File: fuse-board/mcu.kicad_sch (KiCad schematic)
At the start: 33 parts, among them IC1 TMUX1308QPWRQ1, J1 FTSH-107-01-F-DV-K-P-TR, SW1 Y97KT23B5NAFP, U1 STM32G441KBTx, Y1 ECS-240-8-37B-CKY-TR

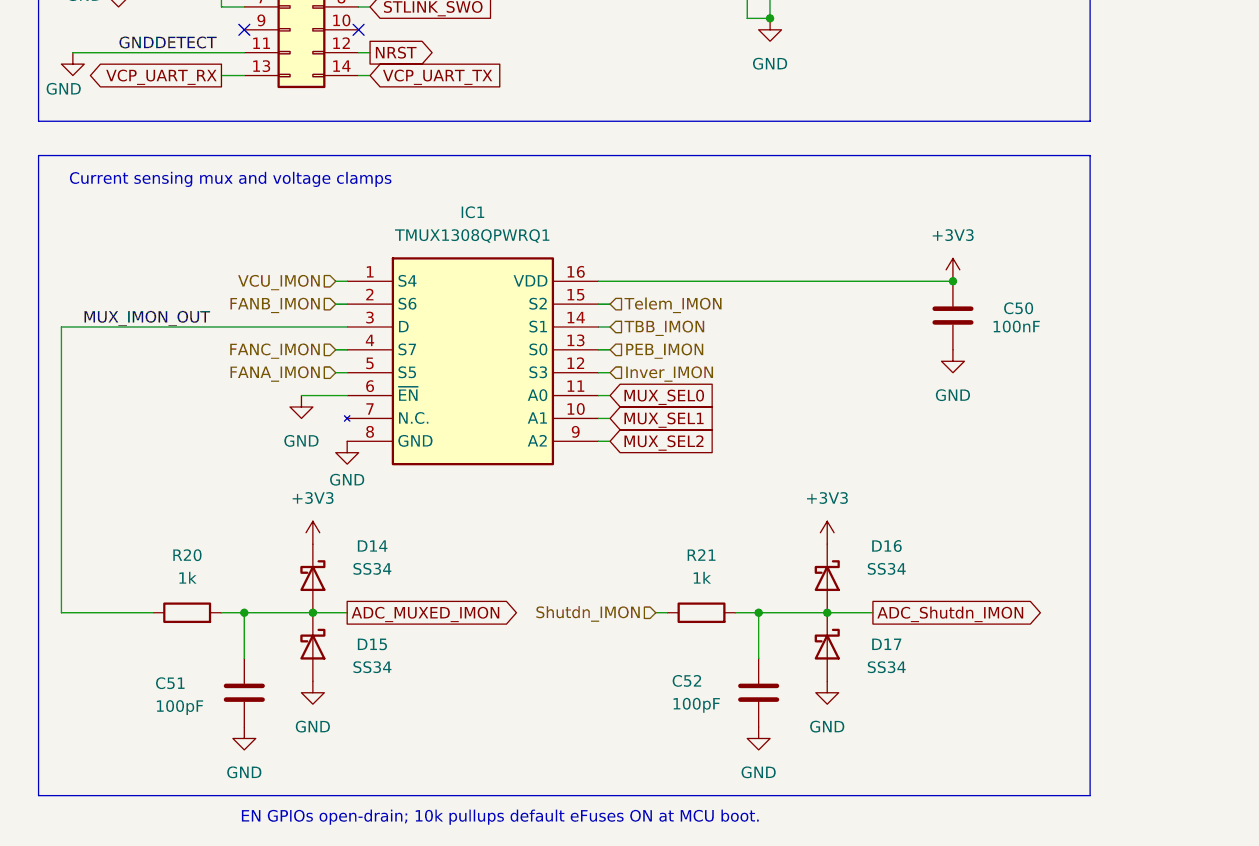
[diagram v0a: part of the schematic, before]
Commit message: update tmux1308
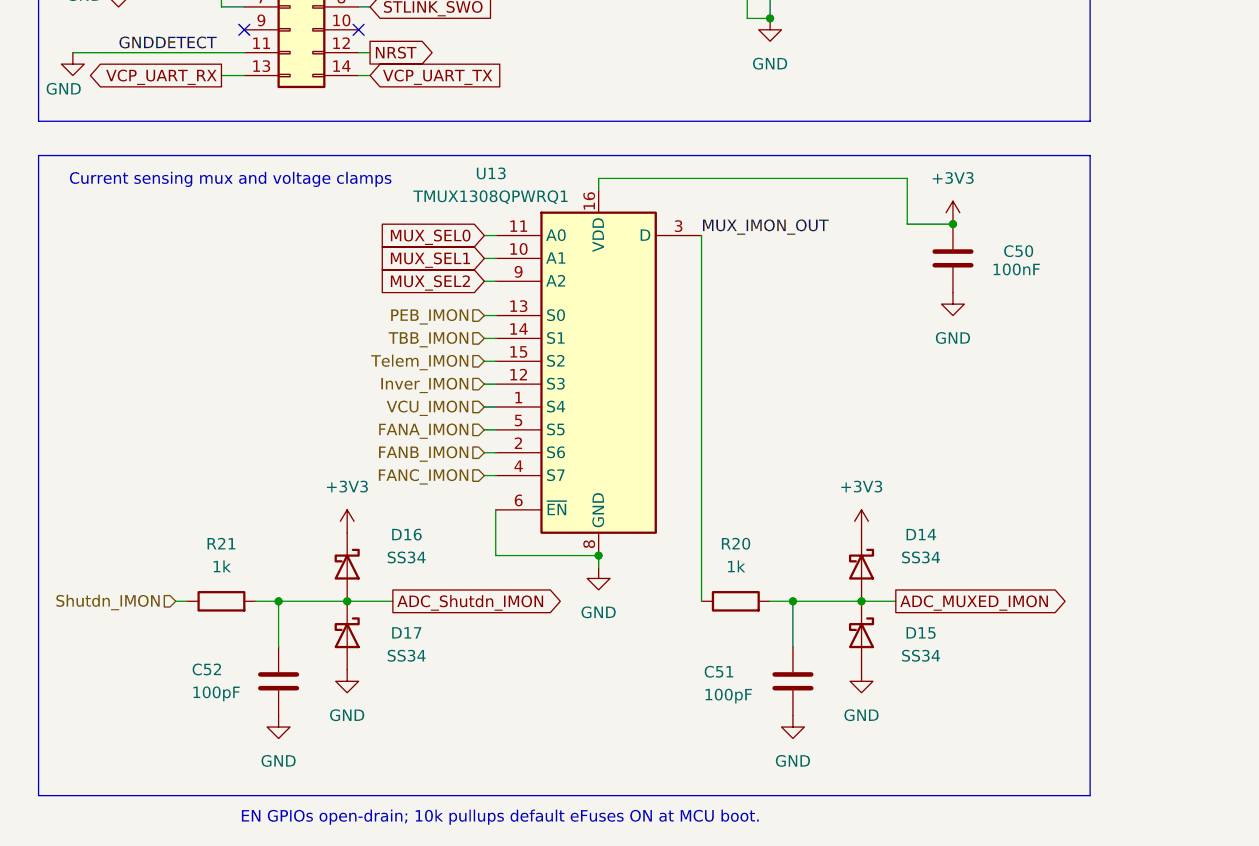
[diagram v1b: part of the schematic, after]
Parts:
- removed IC1: TMUX1308QPWRQ1, formula_slug_footprint_library:SOP65P640X120-16N, symbol formula_slug_symbol_library:TMUX1308QPWRQ1
- added U13: TMUX1308QPWRQ1, formula_slug_footprint_library:SOP65P640X120-16N, symbol formula_slug_symbol_library:TMUX1308QPWRQ1
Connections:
- net +3V3: now also U13.16 (VDD)
- net FANA_IMON: now also U13.5 (S5)
- net FANB_IMON: now also U13.2 (S6)
- net FANC_IMON: now also U13.4 (S7)
- net GND: now also U13.6 (~{EN}), U13.8 (GND)
- net Inver_IMON: now also U13.12 (S3)
- net MUX_IMON_OUT: now also U13.3 (D)
- net MUX_SEL0: now also U13.11 (A0)
- net MUX_SEL1: now also U13.10 (A1)
- net MUX_SEL2: now also U13.9 (A2)
- net PEB_IMON: now also U13.13 (S0)
- net TBB_IMON: now also U13.14 (S1)
- net Telem_IMON: now also U13.15 (S2)
- net VCU_IMON: now also U13.1 (S4)
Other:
- moved on the sheet: C50, C51, C52, D14, D15, D16, D17, R20, R21
